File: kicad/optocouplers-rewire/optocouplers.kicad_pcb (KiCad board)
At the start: 2 copper layers, 123 parts, among them Q1 PN2222A, Q2 PN2222A, Q3 PN2222A, Q4 PN2222A, Q5 PN2222A, Q6 PN2222A, Q7 PN2222A, Q8 PN2222A

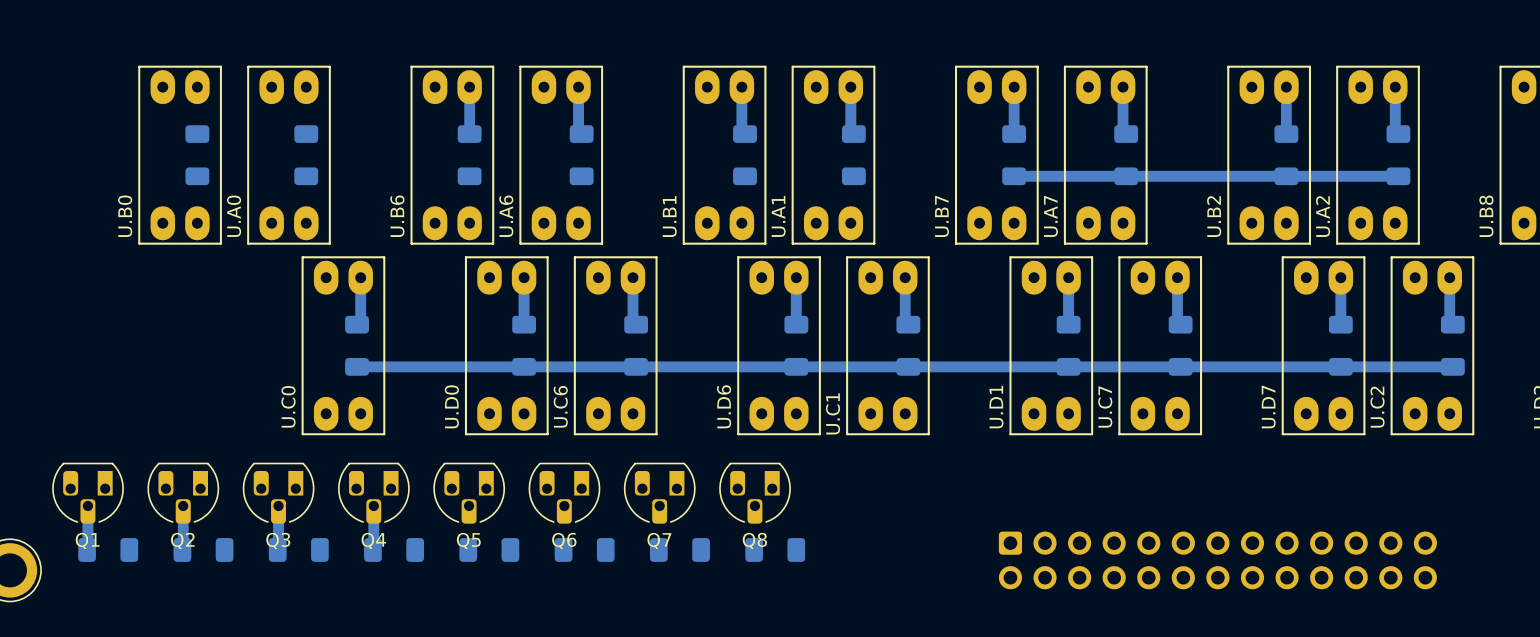
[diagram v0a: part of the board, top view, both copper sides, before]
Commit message: remove segments
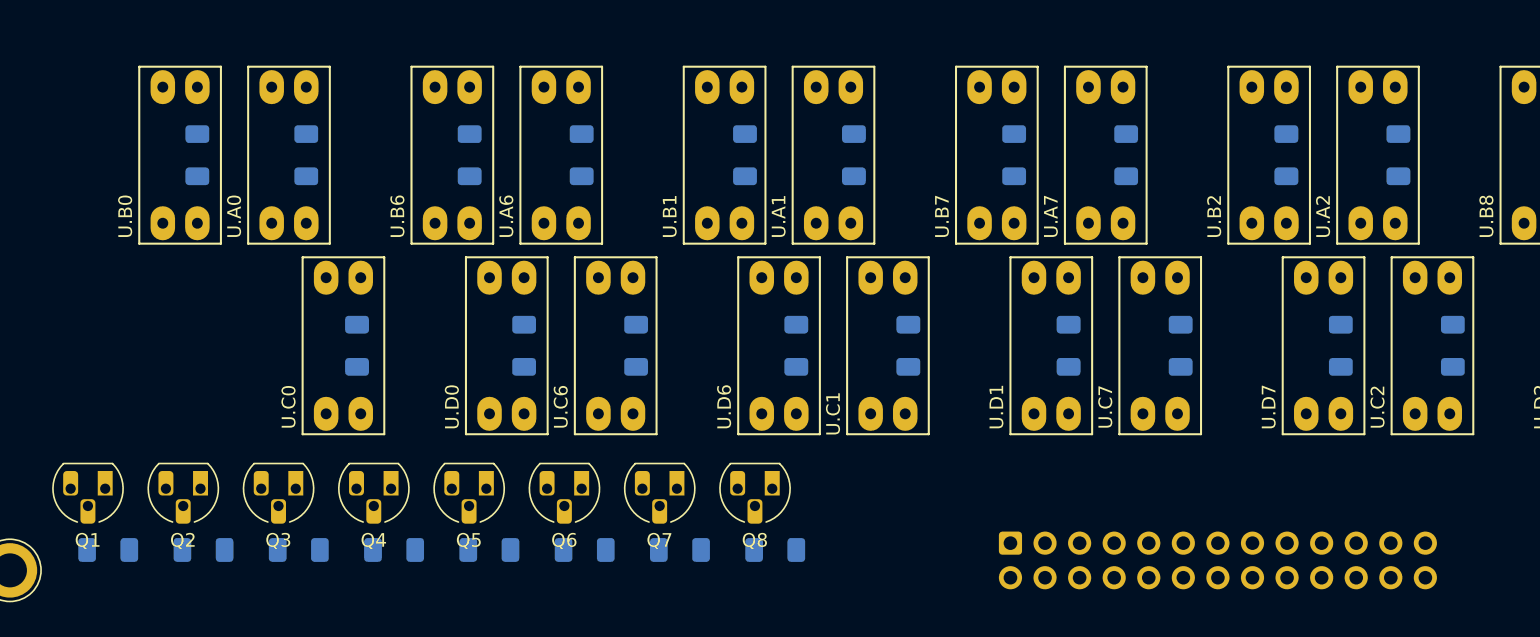
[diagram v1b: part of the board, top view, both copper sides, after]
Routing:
- net +5V: track 108.7 -> 0.00 mm
- net Net-(R.C0-Pad1): track 3.56 -> 0.00 mm
- net Net-(R.C7-Pad1): track 3.55 -> 0.00 mm
- net Net-(R.C2-Pad1): track 3.55 -> 0.00 mm
- net Net-(R.C1-Pad1): track 3.55 -> 0.00 mm
- net Net-(R.A7-Pad1): track 3.55 -> 0.00 mm
- net Net-(R.A2-Pad1): track 3.55 -> 0.00 mm
- net Net-(R.A1-Pad1): track 3.55 -> 0.00 mm
- net Net-(U.A6-Pad1): track 3.55 -> 0.00 mm
- net Net-(R.C6-Pad1): track 3.55 -> 0.00 mm
- net Net-(R.B1-Pad1): track 3.55 -> 0.00 mm
- net Net-(R.D7-Pad1): track 3.45 -> 0.00 mm
- net Net-(R.D6-Pad1): track 3.45 -> 0.00 mm
- net Net-(R.D1-Pad1): track 3.45 -> 0.00 mm
- net Net-(R.D0-Pad1): track 3.45 -> 0.00 mm
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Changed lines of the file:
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@@
     )
   )
-  (segment (start 15.73 63.44) (end 15.67 63.5) (width 0.8) (layer "B.Cu") (net 1))
-  (segment (start 15.73 60.27) (end 15.73 63.44) (width 0.8) (layer "B.Cu") (net 1))
-  (segment (start 76 50.05) (end 116 50.05) (width 0.8) (layer "B.Cu") (net 4))
-  (segment (start 83.77 36.05) (end 112 36.05) (width 0.8) (layer "B.Cu") (net 4))
-  (segment (start 35.5 50.05) (end 76 50.05) (width 0.8) (layer "B.Cu") (net 4))
-  (segment (start 22.73 63.44) (end 22.67 63.5) (width 0.8) (layer "B.Cu") (net 20))
-  (segment (start 22.73 60.27) (end 22.73 63.44) (width 0.8) (layer "B.Cu") (net 20))
-  (segment (start 29.73 63.44) (end 29.67 63.5) (width 0.8) (layer "B.Cu") (net 21))
-  (segment (start 29.73 60.27) (end 29.73 63.44) (width 0.8) (layer "B.Cu") (net 21))
-  (segment (start 36.73 63.44) (end 36.67 63.5) (width 0.8) (layer "B.Cu") (net 24))
-  (segment (start 36.73 60.27) (end 36.73 63.44) (width 0.8) (layer "B.Cu") (net 24))
-  (segment (start 31.77 32.72) (end 32 32.95) (width 0.8) (layer "B.Cu") (net 41))
-  (segment (start 71.77 32.72) (end 72 32.95) (width 0.8) (layer "B.Cu") (net 42))
-  (segment (start 71.77 29.5) (end 71.77 32.72) (width 0.8) (layer "B.Cu") (net 42))
-  (segment (start 111.77 29.5) (end 111.77 32.72) (width 0.8) (layer "B.Cu") (net 43))
-  (segment (start 111.77 32.72) (end 112 32.95) (width 0.8) (layer "B.Cu") (net 43))
-  (segment (start 51.77 32.72) (end 52 32.95) (width 0.8) (layer "B.Cu") (net 47))
-  (segment (start 51.77 29.5) (end 51.77 32.72) (width 0.8) (layer "B.Cu") (net 47))
-  (segment (start 91.77 32.72) (end 92 32.95) (width 0.8) (layer "B.Cu") (net 48))
-  (segment (start 91.77 29.5) (end 91.77 32.72) (width 0.8) (layer "B.Cu") (net 48))
-  (segment (start 23.77 32.72) (end 24 32.95) (width 0.8) (layer "B.Cu") (net 53))
-  (segment (start 63.77 32.72) (end 64 32.95) (width 0.8) (layer "B.Cu") (net 54))
-  (segment (start 63.77 29.5) (end 63.77 32.72) (width 0.8) (layer "B.Cu") (net 54))
-  (segment (start 103.77 29.5) (end 103.77 32.95) (width 0.8) (layer "B.Cu") (net 55))
-  (segment (start 43.77 29.5) (end 43.77 32.95) (width 0.8) (layer "B.Cu") (net 59))
-  (segment (start 83.77 29.5) (end 83.77 32.95) (width 0.8) (layer "B.Cu") (net 60))
-  (segment (start 35.77 43.5) (end 35.77 46.68) (width 0.8) (layer "B.Cu") (net 66))
-  (segment (start 35.77 46.68) (end 35.5 46.95) (width 0.8) (layer "B.Cu") (net 66))
-  (segment (start 75.77 43.5) (end 75.77 46.72) (width 0.8) (layer "B.Cu") (net 67))
-  (segment (start 75.77 46.72) (end 76 46.95) (width 0.8) (layer "B.Cu") (net 67))
-  (segment (start 115.77 46.72) (end 116 46.95) (width 0.8) (layer "B.Cu") (net 68))
-  (segment (start 115.77 43.5) (end 115.77 46.72) (width 0.8) (layer "B.Cu") (net 68))
-  (segment (start 55.77 46.72) (end 56 46.95) (width 0.8) (layer "B.Cu") (net 72))
-  (segment (start 55.77 43.5) (end 55.77 46.72) (width 0.8) (layer "B.Cu") (net 72))
-  (segment (start 95.77 43.5) (end 95.77 46.72) (width 0.8) (layer "B.Cu") (net 73))
-  (segment (start 95.77 46.72) (end 96 46.95) (width 0.8) (layer "B.Cu") (net 73))
-  (segment (start 47.77 43.5) (end 47.77 46.95) (width 0.8) (layer "B.Cu") (net 78))
-  (segment (start 87.77 43.5) (end 87.77 46.95) (width 0.8) (layer "B.Cu") (net 79))
-  (segment (start 67.77 43.5) (end 67.77 46.95) (width 0.8) (layer "B.Cu") (net 84))
-  (segment (start 107.77 43.5) (end 107.77 46.95) (width 0.8) (layer "B.Cu") (net 85))
   (zone (net 3) (net_name "GND") (layer "F.Cu") (hatch edge 0.508)
     (connect_pads (clearance 0.508))
